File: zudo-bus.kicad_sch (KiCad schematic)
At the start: 17 parts, among them P1 WJ500V-5.08-2P-14-00A, P2 WJ500V-5.08-2P-14-00A, U1 AMS1117-5.0

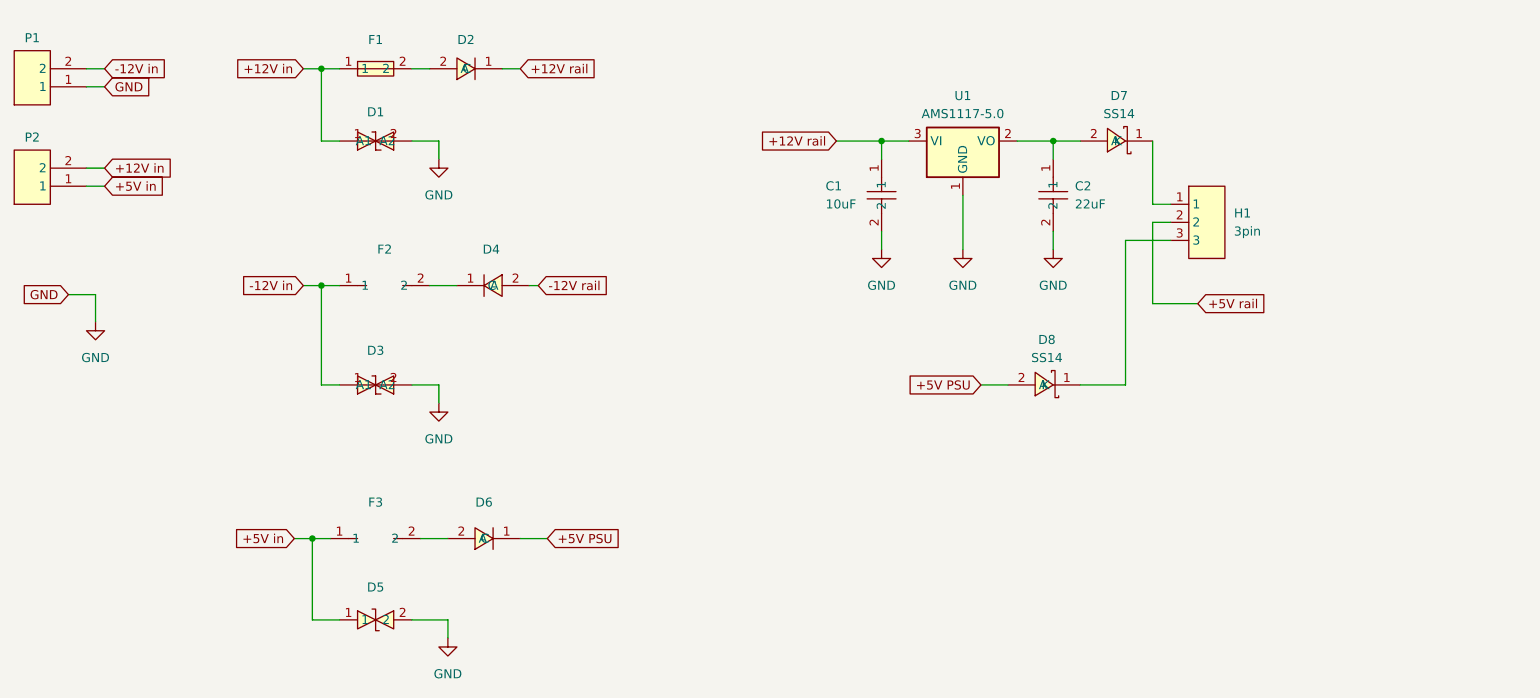
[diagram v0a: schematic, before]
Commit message: wip
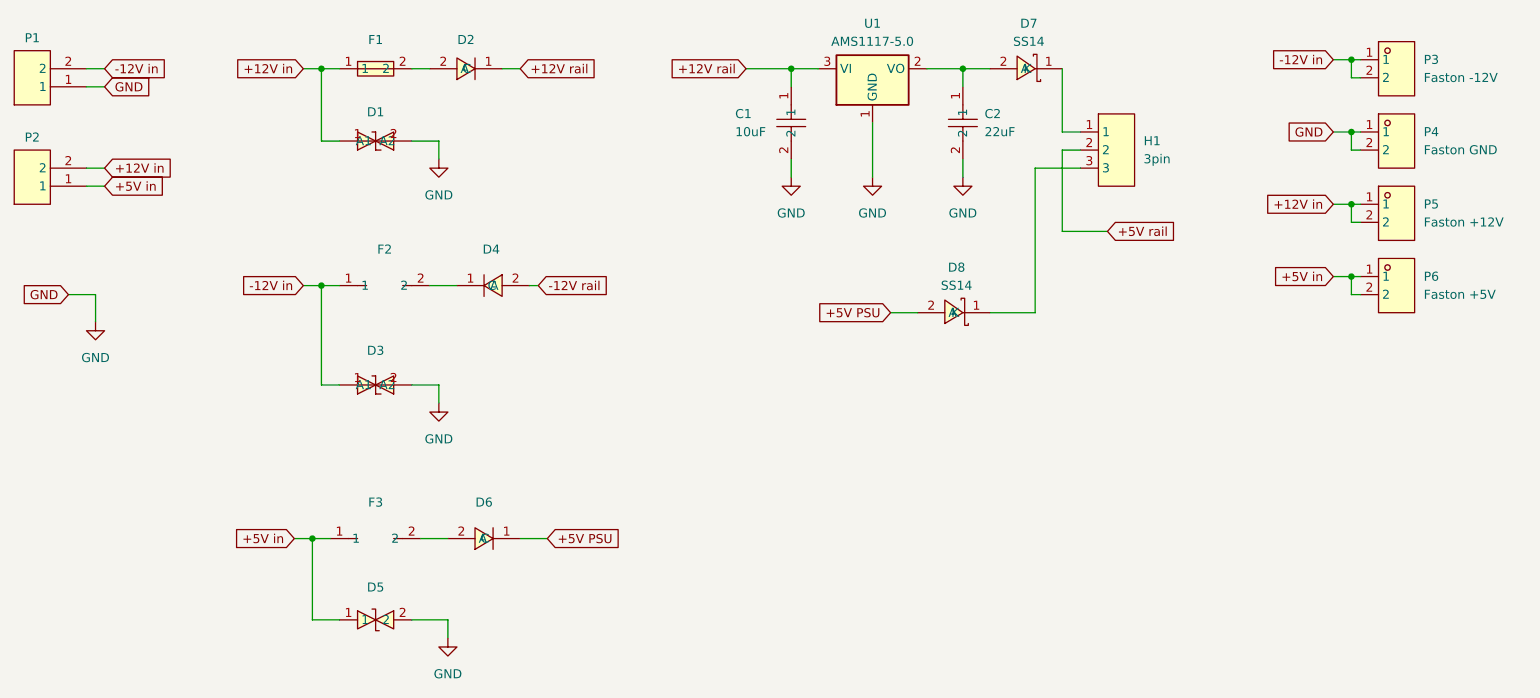
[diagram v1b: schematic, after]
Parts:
- added P3: Faston -12V, easyeda2kicad:CONN-TH_1217754-1, symbol zudo-bus:1217754-1
- added P4: Faston GND, easyeda2kicad:CONN-TH_1217754-1, symbol zudo-bus:1217754-1
- added P5: Faston +12V, easyeda2kicad:CONN-TH_1217754-1, symbol zudo-bus:1217754-1
- added P6: Faston +5V, easyeda2kicad:CONN-TH_1217754-1, symbol zudo-bus:1217754-1
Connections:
- net +12V in: now also P5.1, P5.2
- net +5V in: now also P6.1, P6.2
- net -12V in: now also P3.1, P3.2
- net GND: now also P4.1, P4.2
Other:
- moved on the sheet: C1, C2, D7, D8, H1, U1
